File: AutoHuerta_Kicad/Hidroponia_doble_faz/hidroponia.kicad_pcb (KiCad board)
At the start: 2 copper layers, 37 parts, among them J1 bornera, J2 bornera, J3 Barrel_Jack, J4 pin, J6 Pin, J7 Pin, K1 RELAY, Q1 BC817, Q2 BS170F, Q3 BC817, U2 PC817, U3 L7805, U4 PC817, U5 L7805, U6 PC817

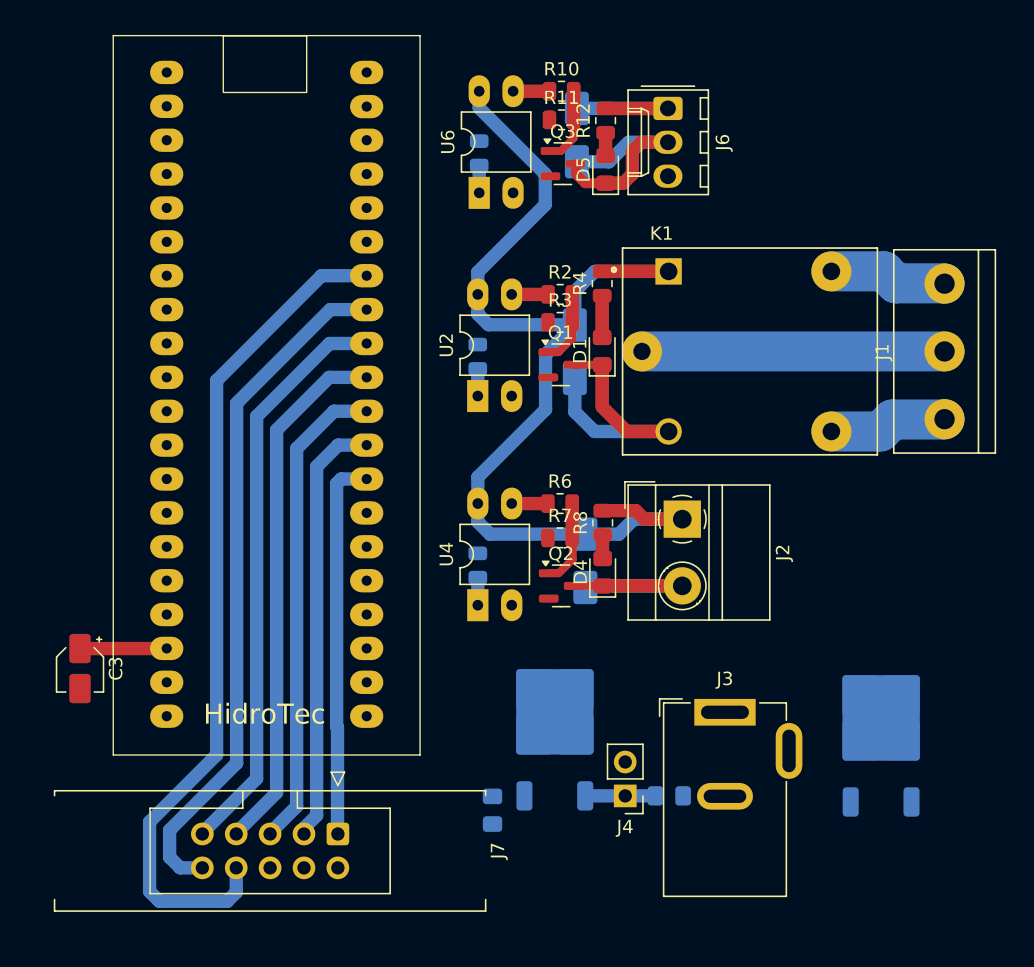
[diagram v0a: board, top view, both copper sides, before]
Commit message: PCB TERMINADO
Terminamos el PCB
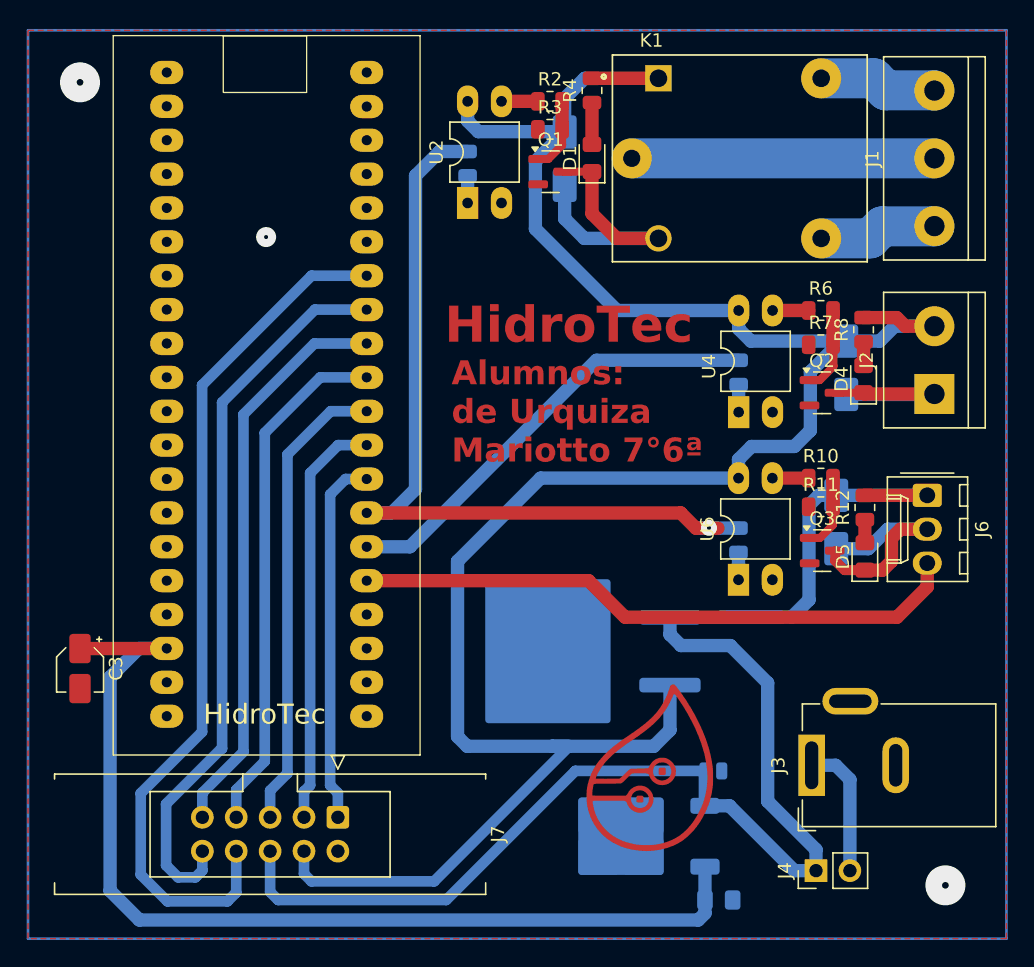
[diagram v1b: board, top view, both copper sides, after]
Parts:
- added G***: LOGO, Huellas:Logo, F.Cu at (81.5, 88.4)
- C1: footprint Capacitor_SMD:C_0805_2012Metric_Pad1.18x1.45mm_HandSolder -> Capacitor_SMD:C_0504_1310Metric_Pad0.83x1.28mm_HandSolder
- J2: footprint TerminalBlock_MetzConnect:TerminalBlock_MetzConnect_Type011_RT05502HBWC_1x02_P5.00mm_Horizontal -> TerminalBlock:TerminalBlock_bornier-2_P5.08mm
- U5: footprint Package_TO_SOT_SMD:TO-252-2 -> Package_TO_SOT_SMD:TO-263-2_TabPin1
- moved R10 34.9 mm to (94.3, 66.6)
- moved R11 34.9 mm to (94.3, 68.7)
- moved R12 34.9 mm to (97.6, 68.8)
- moved R9 34.9 mm to (88.1, 71.2)
- moved D5 34.9 mm to (97.6, 72.4)
- moved D6 34.9 mm to (95.4, 69.9)
- moved J6 34.9 mm to (102.3, 67.9)
- moved Q3 34.9 mm to (94.4, 72.0)
- moved U6 34.9 mm to (88.1, 74.2)
- moved D3 24.3 mm to (96.2, 58.3)
- moved Q2 24.3 mm to (94.4, 60.2)
- moved D4 24.3 mm to (97.5, 59.1)
- moved R5 24.3 mm to (88.1, 58.6)
- moved R6 24.3 mm to (94.3, 54.0)
- moved R7 24.3 mm to (94.3, 56.6)
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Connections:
- J2 pad 1: +5V -> Net-(D3-A)
- J2 pad 2: Net-(D3-A) -> +5V
- U1 pad 25: LED & FAN -> VEL
- U1 pad 26: VEL -> BOMBA
- U1 pad 27: BOMBA -> LED & FAN
- U5 pad 1: +12V -> GND
- U5 pad 2: GND -> +5V
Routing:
- net +12V: track 16.8 -> 119.0 mm
- net +5V: track 83.8 -> 172.6 mm
- net +5V1: track 6.50 -> 76.9 mm
- net LED & FAN: track 0.00 -> 63.4 mm, vias 0 -> 1
- net VEL: track 0.00 -> 45.9 mm
- net BOMBA: track 0.00 -> 33.7 mm
- net Net-(J4-Pin_2): track 0.00 -> 10.1 mm
- net B0: track 51.6 -> 54.9 mm
- net B1: track 63.8 -> 65.7 mm
- net A4: track 32.4 -> 31.1 mm
- net A5: track 36.1 -> 35.0 mm
- net A3: track 28.7 -> 27.7 mm
- net Net-(D3-A): track 15.5 -> 14.5 mm
- net A6: track 39.9 -> 39.1 mm
- net A7: track 43.5 -> 42.9 mm
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- added copper zone on B.Cu, net GND
- added copper zone on F.Cu, net GND
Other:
- board text added: "Alumnos: de Urquiza Mariotto 7°6ª"
- board text added: "HidroTec"
